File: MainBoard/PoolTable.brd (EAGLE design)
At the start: 457.2 x 166 mm, 77 parts, among them IC1 LM317MBSTT3, IC2 LM317MBSTT3, IC3 LM317MBSTT3, IC5 MIC2026-1YM, IC7 AP2331W-7, J1 USB_A_SMT_FEMALE, J2 USB_A_SMT_FEMALE, J4 SD_CARD_SOCKET, Q1 DMG1012T-7, Q2 DMG1012T-7, Q3 DMG1012T-7, U1 TMP102, U2 TMP102, U3 TMP102, U4 TMP102, U5 LAN9512-JZX, U6 FSUSB42UMX

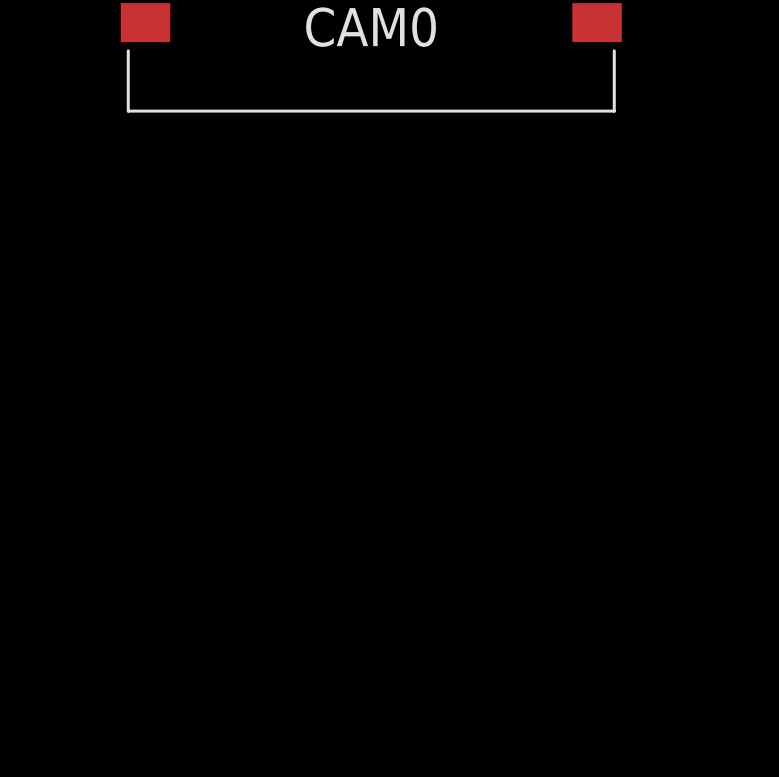
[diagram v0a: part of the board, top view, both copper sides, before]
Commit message: First HDMI work
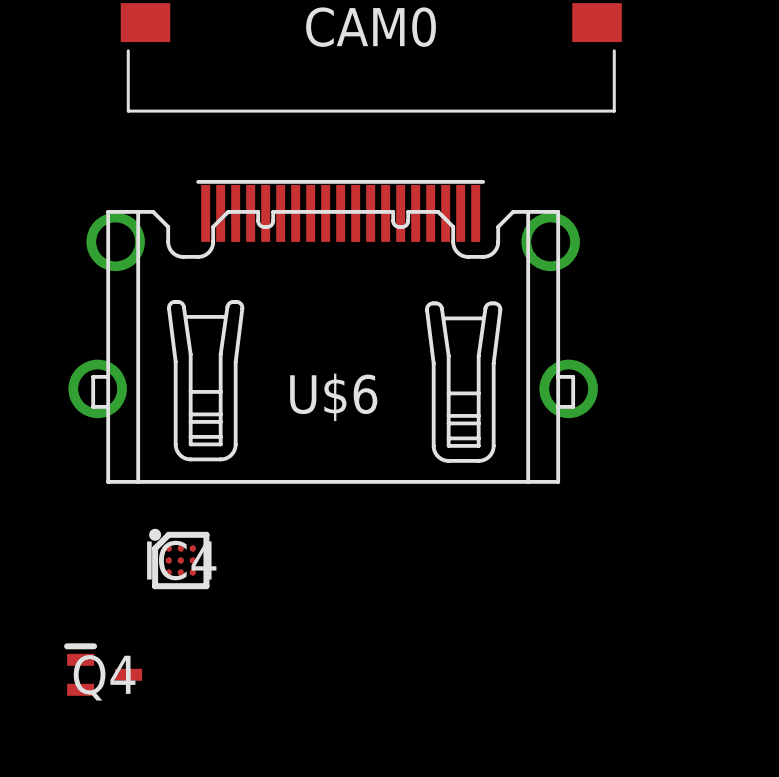
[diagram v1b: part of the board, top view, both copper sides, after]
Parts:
- added IC4: ESD5384NCTBG, SamacSys_Parts:BGA9C40P3X3_114X114X63
- added Q4: DMG1012T-7, SamacSys_Parts:SOT50P160X80-3N
- added U$6: HDMI-A, connectors:HDMI_A
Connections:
- new net N$4: IC4.A3, U$6.P$15
- new net N$5: IC4.B3, U$6.P$16
- new net N$7: IC4.A2, Q4.2, U$6.P$13
- new net N$8: IC4.C3, U$6.P$19
- net GND: now also IC4.B2, IC4.C2, U$6.P$11, U$6.P$17, U$6.P$2, U$6.P$5, U$6.P$8
- net H5V: now also IC4.A1, IC4.C1, Q4.1, U$6.P$18
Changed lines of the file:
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@@
 <?xml version="1.0" encoding="utf-8"?>
 <!DOCTYPE eagle SYSTEM "eagle.dtd">
-<eagle version="9.3.0">
+<eagle version="9.2.2">
 <drawing>
 <settings>
@@
 <attribute name="VALUE" x="-52.07" y="-450.85" size="1.27" layer="27" align="center"/>
 </element>
+<element name="U$6" library="connectors" package="HDMI_A" value="HDMI-A" x="-53.34" y="-461.01" smashed="yes">
+<attribute name="NAME" x="-53.34" y="-463.09" size="1.27" layer="25" font="vector" align="center"/>
+</element>
+<element name="IC4" library="SamacSys_Parts" package="BGA9C40P3X3_114X114X63" value="ESD5384NCTBG" x="-58.42" y="-468.63" smashed="yes">
+<attribute name="DESCRIPTION" value="" x="-58.42" y="-468.63" size="1.778" layer="27" display="off"/>
+<attribute name="HEIGHT" value="0.63mm" x="-58.42" y="-468.63" size="1.778" layer="27" display="off"/>
+<attribute name="MANUFACTURER_NAME" value="ON Semiconductor" x="-58.42" y="-468.63" size="1.778" layer="27" display="off"/>
+<attribute name="MANUFACTURER_PART_NUMBER" value="ESD5384NCTBG" x="-58.42" y="-468.63" size="1.778" layer="27" display="off"/>
+<attribute name="MOUSER_PART_NUMBER" value="863-ESD5384NCTBG" x="-58.42" y="-468.63" size="1.778" layer="27" display="off"/>
+<attribute name="NAME" x="-58.42" y="-468.63" size="1.27" layer="25" align="center"/>
+<attribute name="VALUE" x="-58.42" y="-468.63" size="1.27" layer="27" align="center"/>
+</element>
+<element name="Q4" library="SamacSys_Parts" package="SOT50P160X80-3N" value="DMG1012T-7" x="-60.96" y="-472.44" smashed="yes">
+<attribute name="DESCRIPTION" value="MOSFET N-Channel 20V 0.63A SOT523 Diodes Inc DMG1012T-7 N-channel MOSFET Transistor, 0.63 A, 20 V, 3-Pin SOT-523" x="-60.96" y="-472.44" size="1.778" layer="27" display="off"/>
+<attribute name="HEIGHT" value="0.8mm" x="-60.96" y="-472.44" size="1.778" layer="27" display="off"/>
+<attribute name="MANUFACTURER_NAME" value="Diodes Inc." x="-60.96" y="-472.44" size="1.778" layer="27" display="off"/>
+<attribute name="MANUFACTURER_PART_NUMBER" value="DMG1012T-7" x="-60.96" y="-472.44" size="1.778" layer="27" display="off"/>
+<attribute name="MOUSER_PART_NUMBER" value="621-DMG1012T-7" x="-60.96" y="-472.44" size="1.778" layer="27" display="off"/>
+<attribute name="NAME" x="-60.96" y="-472.44" size="1.27" layer="25" align="center"/>
+<attribute name="VALUE" x="-60.96" y="-472.44" size="1.27" layer="27" align="center"/>
+</element>
 </elements>
 <signals>
@@
 <contactref element="CAM0" pad="23"/>
 <contactref element="CAM0" pad="24"/>
+<contactref element="IC4" pad="C2"/>
+<contactref element="IC4" pad="B2"/>
+<contactref element="U$6" pad="P$2"/>
+<contactref element="U$6" pad="P$5"/>
+<contactref element="U$6" pad="P$8"/>
+<contactref element="U$6" pad="P$11"/>
+<contactref element="U$6" pad="P$17"/>
+<wire x1="-50.59" y1="-457.06" x2="-52.09" y2="-457.06" width="0" layer="19" extent="1-1"/>
+<wire x1="-49.09" y1="-457.06" x2="-50.59" y2="-457.06" width="0" layer="19" extent="1-1"/>
+<wire x1="-53.59" y1="-457.06" x2="-52.09" y2="-457.06" width="0" layer="19" extent="1-1"/>
+<wire x1="-56.59" y1="-457.06" x2="-53.59" y2="-457.06" width="0" layer="19" extent="1-1"/>
+<wire x1="-59.595" y1="-450.7" x2="-56.59" y2="-457.06" width="0" layer="19" extent="1-1"/>
+<wire x1="-57.32" y1="-448.8" x2="-59.595" y2="-450.7" width="0" layer="19" extent="1-1"/>
 <wire x1="-55.82" y1="-448.8" x2="-57.32" y2="-448.8" width="0" layer="19" extent="1-1"/>
 <wire x1="-54.32" y1="-448.8" x2="-55.82" y2="-448.8" width="0" layer="19" extent="1-1"/>
@@
 <wire x1="-49.82" y1="-448.8" x2="-51.32" y2="-448.8" width="0" layer="19" extent="1-1"/>
 <wire x1="-48.32" y1="-448.8" x2="-49.82" y2="-448.8" width="0" layer="19" extent="1-1"/>
-<wire x1="-59.595" y1="-450.7" x2="-57.32" y2="-448.8" width="0" layer="19" extent="1-1"/>
 <wire x1="-44.545" y1="-450.7" x2="-48.32" y2="-448.8" width="0" layer="19" extent="1-1"/>
 <wire x1="-59.595" y1="-441.81" x2="-57.32" y2="-448.8" width="0" layer="19" extent="1-1"/>
@@
 <wire x1="-60.69" y1="-400.7" x2="-58.84" y2="-411.48" width="0" layer="19" extent="1-1"/>
 <wire x1="-60.69" y1="-392.45" x2="-60.69" y2="-400.7" width="0" layer="19" extent="1-1"/>
+<wire x1="-58.42" y1="-468.63" x2="-56.59" y2="-457.06" width="0" layer="19" extent="1-1"/>
+<wire x1="-58.42" y1="-469.03" x2="-58.42" y2="-468.63" width="0" layer="19" extent="1-1"/>
 <wire x1="-61.54" y1="-377.19" x2="-60.69" y2="-392.45" width="0" layer="19" extent="1-1"/>
 <wire x1="-56.57" y1="-377.19" x2="-61.54" y2="-377.19" width="0" layer="19" extent="1-1"/>
@@
 <contactref element="IC7" pad="2"/>
 <contactref element="C15" pad="1"/>
+<contactref element="U$6" pad="P$18"/>
+<contactref element="IC4" pad="C1"/>
+<contactref element="IC4" pad="A1"/>
+<contactref element="Q4" pad="1"/>
 <wire x1="-57.73" y1="-377.19" x2="-58.45" y2="-374.33" width="0" layer="19" extent="1-1"/>
+<wire x1="-57.09" y1="-457.06" x2="-57.73" y2="-377.19" width="0" layer="19" extent="1-1"/>
+<wire x1="-58.82" y1="-468.23" x2="-57.09" y2="-457.06" width="0" layer="19" extent="1-1"/>
+<wire x1="-58.82" y1="-469.03" x2="-58.82" y2="-468.23" width="0" layer="19" extent="1-1"/>
+<wire x1="-61.76" y1="-471.94" x2="-58.82" y2="-469.03" width="0" layer="19" extent="1-1"/>
 </signal>
 <signal name="CPU1_USB_D_P" class="1">
@@
 <contactref element="CAM0" pad="18"/>
 </signal>
+<signal name="N$4">
+<contactref element="IC4" pad="A3"/>
+<contactref element="U$6" pad="P$15"/>
+<wire x1="-55.59" y1="-457.06" x2="-58.02" y2="-468.23" width="0" layer="19" extent="1-1"/>
+</signal>
+<signal name="N$5">
+<contactref element="IC4" pad="B3"/>
+<contactref element="U$6" pad="P$16"/>
+<wire x1="-56.09" y1="-457.06" x2="-58.02" y2="-468.63" width="0" layer="19" extent="1-1"/>
+</signal>
+<signal name="N$8">
+<contactref element="IC4" pad="C3"/>
+<contactref element="U$6" pad="P$19"/>
+<wire x1="-57.59" y1="-457.06" x2="-58.02" y2="-469.03" width="0" layer="19" extent="1-1"/>
+</signal>
+<signal name="N$7">
+<contactref element="IC4" pad="A2"/>
+<contactref element="U$6" pad="P$13"/>
+<contactref element="Q4" pad="2"/>
+<wire x1="-58.42" y1="-468.23" x2="-61.76" y2="-472.94" width="0" layer="19" extent="1-1"/>
+<wire x1="-54.59" y1="-457.06" x2="-58.42" y2="-468.23" width="0" layer="19" extent="1-1"/>
+</signal>
 </signals>
